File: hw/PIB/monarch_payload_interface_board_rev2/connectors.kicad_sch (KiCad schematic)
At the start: 19 parts, among them J1 2200980271, J13 2200980471, J14 2200980471, J15 2200980471, J16 2200980271, J18 2200980671, J19 2200980671, J2 Conn_01x06, J20 2200980671, J21 2200980671, J22 2200980671, J23 2200980671, J24 2200980671, J25 2200980471, J3 Conn_01x05, J4 Conn_01x04, J5 Conn_01x05, J6 2200980671, J8 2200980671

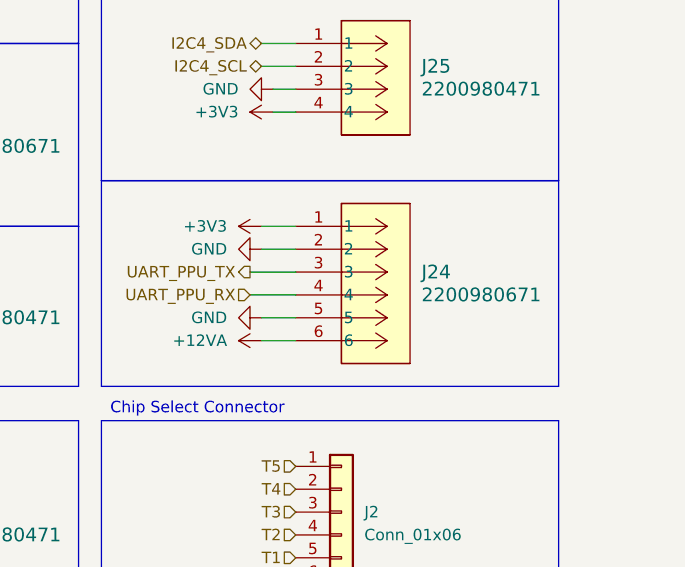
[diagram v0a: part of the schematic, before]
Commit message: Initial Routing Work + Placement
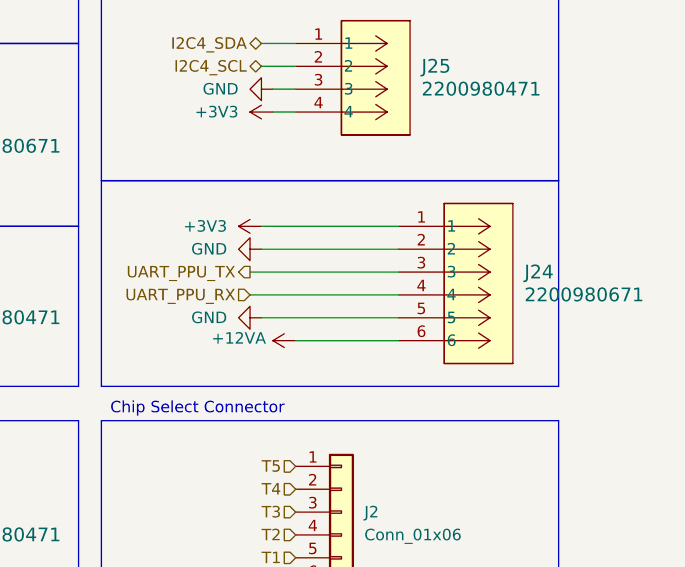
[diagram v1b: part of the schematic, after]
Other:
- moved on the sheet: J24
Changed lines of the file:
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@@
 	(wire
 		(pts
-			(xy 242.57 63.5) (xy 247.65 63.5)
+			(xy 242.57 63.5) (xy 259.08 63.5)
 		)
 		(stroke
@@
 	(wire
 		(pts
+			(xy 259.08 71.12) (xy 247.65 71.12)
+		)
+		(stroke
+			(width 0)
+			(type default)
+		)
+	)
+	(wire
+		(pts
 			(xy 185.42 92.71) (xy 194.31 92.71)
 		)
@@
 	(wire
 		(pts
-			(xy 243.84 68.58) (xy 247.65 68.58)
+			(xy 243.84 68.58) (xy 259.08 68.58)
 		)
 		(stroke
@@
 	(wire
 		(pts
-			(xy 243.84 71.12) (xy 247.65 71.12)
-		)
-		(stroke
-			(width 0)
-			(type default)
-		)
-	)
-	(wire
-		(pts
 			(xy 33.02 52.07) (xy 41.91 52.07)
 		)
@@
 	(wire
 		(pts
-			(xy 243.84 58.42) (xy 247.65 58.42)
+			(xy 243.84 58.42) (xy 259.08 58.42)
 		)
 		(stroke
@@
 	(wire
 		(pts
-			(xy 242.57 66.04) (xy 247.65 66.04)
+			(xy 242.57 66.04) (xy 259.08 66.04)
 		)
 		(stroke
@@
 	(wire
 		(pts
-			(xy 243.84 60.96) (xy 247.65 60.96)
+			(xy 243.84 60.96) (xy 259.08 60.96)
 		)
 		(stroke
@@
 		(lib_name "5037630691_1")
 		(lib_id "5037630691:5037630691")
-		(at 247.65 58.42 0)
+		(at 259.08 58.42 0)
 		(unit 1)
 		(body_style 1)
@@
 		(fields_autoplaced yes)
 		(property "Reference" "J24"
-			(at 261.62 63.4999 0)
+			(at 273.05 63.4999 0)
 			(show_name no)
 			(do_not_autoplace no)
@@
 		)
 		(property "Value" "2200980671"
-			(at 261.62 66.0399 0)
+			(at 273.05 66.0399 0)
 			(show_name no)
 			(do_not_autoplace no)
@@
 		)
 		(property "Footprint" "Connector_Molex_Micro-Lock-Plus:Molex_Micro-Lock_2200980671_1x06_P1.25mm_Horizontal"
-			(at 247.65 58.42 0)
+			(at 259.08 58.42 0)
 			(hide yes)
 			(show_name no)
@@
 		)
 		(property "Datasheet" "https://www.molex.com/en-us/products/part-detail/2200980671"
-			(at 247.65 58.42 0)
+			(at 259.08 58.42 0)
 			(hide yes)
 			(show_name no)
@@
 		)
 		(property "Description" ""
-			(at 247.65 58.42 0)
+			(at 259.08 58.42 0)
 			(hide yes)
 			(show_name no)
@@
 	(symbol
 		(lib_id "power:+12VA")
-		(at 243.84 71.12 90)
+		(at 247.65 71.12 90)
 		(mirror x)
 		(unit 1)
@@
 		(in_pos_files yes)
 		(dnp no)
-		(fields_autoplaced yes)
 		(property "Reference" "#PWR0186"
-			(at 247.65 71.12 0)
+			(at 251.46 71.12 0)
 			(hide yes)
 			(show_name no)
@@
 		)
 		(property "Value" "+12VA"
-			(at 240.03 71.1201 90)
+			(at 244.348 70.866 90)
 			(show_name no)
 			(do_not_autoplace no)
@@
 		)
 		(property "Footprint" ""
-			(at 243.84 71.12 0)
+			(at 247.65 71.12 0)
 			(hide yes)
 			(show_name no)
@@
 		)
 		(property "Datasheet" ""
-			(at 243.84 71.12 0)
+			(at 247.65 71.12 0)
 			(hide yes)
 			(show_name no)
@@
 		)
 		(property "Description" "Power symbol creates a global label with name \"+12VA\""
-			(at 243.84 71.12 0)
+			(at 247.65 71.12 0)
 			(hide yes)
 			(show_name no)
